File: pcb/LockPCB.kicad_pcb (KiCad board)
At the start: 4 copper layers, 17.5 x 60 mm, 0 parts

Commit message: Record recommended blocker defaults and review envelope
Co-authored-by: arena-agent <297053741+arena-agent@users.noreply.github.com>
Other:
- board text added: "20 x 65 mm REVIEW ENVELOPE - PROPOSED / TBD"
- board text removed: "17.5 x 60 mm - PLACEHOLDER"
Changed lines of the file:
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@@
   (gr_text "BATTERY_CONTACT_ZONE" (at -2.8 21.5 0) (layer "User.2") (effects (font (size 0.62 0.62) (thickness 0.1))))
   (gr_text "CONTACT / POLARITY TBD" (at -2.8 39 0) (layer "User.2") (effects (font (size 0.56 0.56) (thickness 0.09))))
-  (gr_rect (start 0 0) (end 17.5 60) (stroke (width 0.12) (type dash)) (fill none) (layer "User.3"))
+  (gr_rect (start -1.25 -2.5) (end 18.75 62.5) (stroke (width 0.12) (type dash)) (fill none) (layer "User.3"))
   (gr_text "PCB_MAX_OUTLINE" (at 1.0 2.0 0) (layer "User.3") (effects (font (size 0.72 0.72) (thickness 0.11))))
-  (gr_text "17.5 x 60 mm - PLACEHOLDER" (at 1.0 4.0 0) (layer "User.3") (effects (font (size 0.58 0.58) (thickness 0.09))))
+  (gr_text "20 x 65 mm REVIEW ENVELOPE - PROPOSED / TBD" (at 1.0 4.0 0) (layer "User.3") (effects (font (size 0.58 0.58) (thickness 0.09))))
   (gr_rect (start -1 -10) (end 18.5 8) (stroke (width 0.2) (type dash)) (fill none) (layer "User.4"))
   (gr_text "MOTOR_GEARBOX_ZONE" (at -0.2 -8.2 0) (layer "User.4") (effects (font (size 0.72 0.72) (thickness 0.11))))

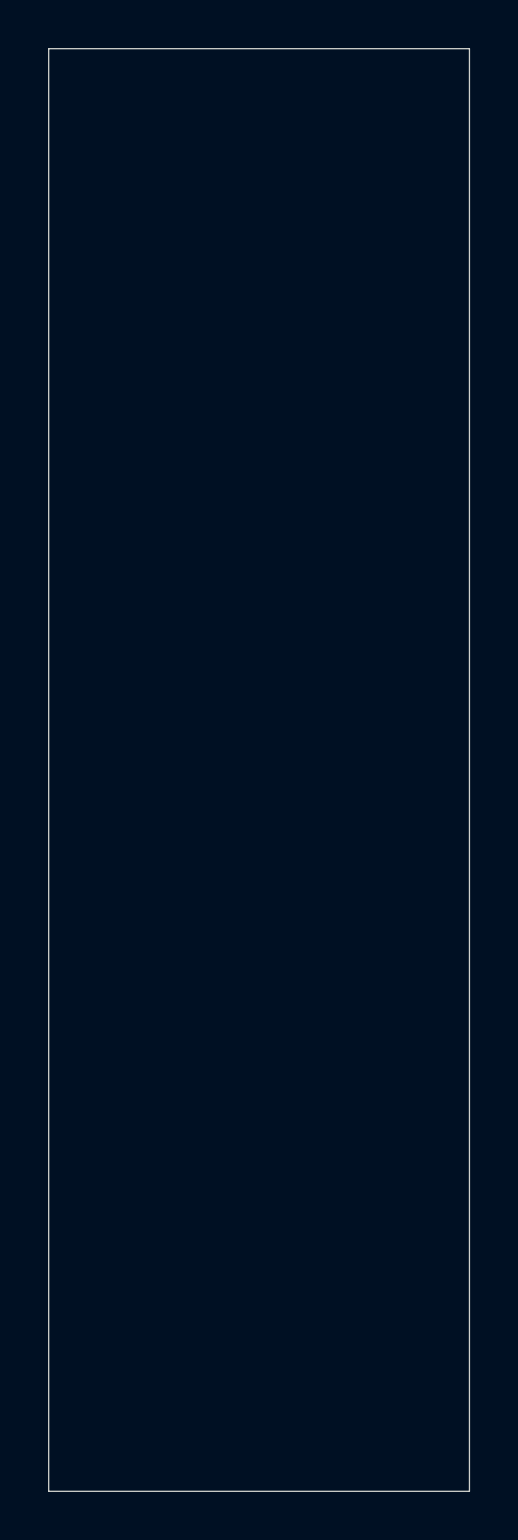
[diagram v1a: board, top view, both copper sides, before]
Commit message: Align agent PCB outline to confirmed prototype CAD
Co-authored-by: arena-agent <297053741+arena-agent@users.noreply.github.com>
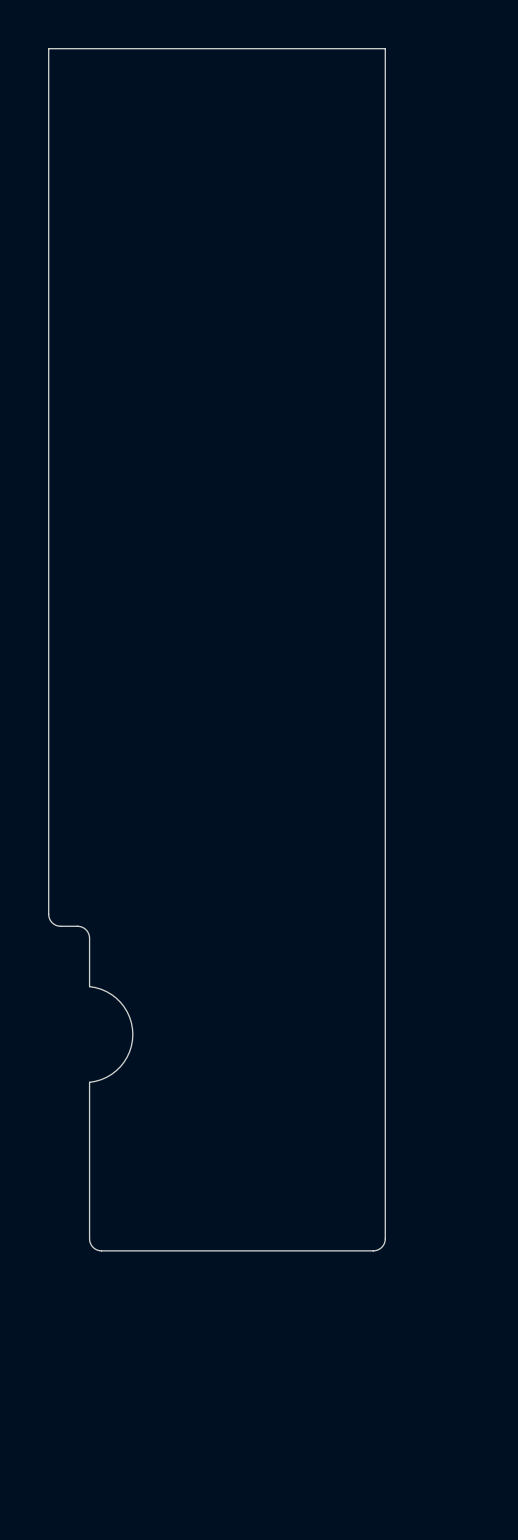
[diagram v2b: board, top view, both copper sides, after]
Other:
- board size 17.5 x 60 mm -> 14 x 50 mm
- board text added: "2x D3.1 / D5 RINGS; PADS / POLARITY TBD"
- board text added: "4-CU PREFERENCE; DWG THICKNESS CALLOUT 1.20 mm; STACKUP TBD"
- board text added: "CELL SKU / CONTACT PAD IMPLEMENTATION / MOTOR DATA / FINAL FIT: TBD"
- board text added: "DESIGNER DWG: 14 x 50 mm; NO EXTRA MARGIN SPECIFIED"
- board text added: "DWG-DERIVED EDGE / HOLE REFERENCES; AGENT ZONES STILL PROVISIONAL - NOT FOR FABRICATION"
- board text added: "PCB_MAX_OUTLINE - SOURCE EXTENT"
- board text added: "STEP 18x50 AABB; ORIENTATION / CLEARANCE TBD"
- board text removed: "18650 SIZE, MOTOR DATA, BODY FIT, CLEARANCES: TBD"
- board text removed: "20 x 65 mm REVIEW ENVELOPE - PROPOSED / TBD"
- board text removed: "4-CU STARTING PREFERENCE; PCB THICKNESS / COPPER WEIGHT: TBD"
- board text removed: "CONTACT / POLARITY TBD"
- board text removed: "MECHANICAL PLACEHOLDERS - NOT TO SCALE - NOT FOR FABRICATION"
- board text removed: "PCB_MAX_OUTLINE"
- board text removed: "TBD / NTS"
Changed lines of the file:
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@@
     (58 "User.9" user)
   )
-  (gr_line (start 0 0) (end 17.5 0) (stroke (width 0.05) (type default)) (layer "Edge.Cuts"))
-  (gr_line (start 17.5 0) (end 17.5 60) (stroke (width 0.05) (type default)) (layer "Edge.Cuts"))
-  (gr_line (start 17.5 60) (end 0 60) (stroke (width 0.05) (type default)) (layer "Edge.Cuts"))
-  (gr_line (start 0 60) (end 0 0) (stroke (width 0.05) (type default)) (layer "Edge.Cuts"))
-  (gr_rect (start -21 1) (end -1 59) (stroke (width 0.18) (type dash)) (fill none) (layer "User.1"))
-  (gr_text "BATTERY_KEEP_OUT" (at -20 0 0) (layer "User.1") (effects (font (size 0.72 0.72) (thickness 0.11))))
-  (gr_text "TBD / NTS" (at -19 3 0) (layer "User.1") (effects (font (size 0.65 0.65) (thickness 0.1))))
-  (gr_rect (start -3 23) (end 0.5 37) (stroke (width 0.2) (type dash)) (fill none) (layer "User.2"))
-  (gr_text "BATTERY_CONTACT_ZONE" (at -2.8 21.5 0) (layer "User.2") (effects (font (size 0.62 0.62) (thickness 0.1))))
-  (gr_text "CONTACT / POLARITY TBD" (at -2.8 39 0) (layer "User.2") (effects (font (size 0.56 0.56) (thickness 0.09))))
-  (gr_rect (start -1.25 -2.5) (end 18.75 62.5) (stroke (width 0.12) (type dash)) (fill none) (layer "User.3"))
-  (gr_text "PCB_MAX_OUTLINE" (at 1.0 2.0 0) (layer "User.3") (effects (font (size 0.72 0.72) (thickness 0.11))))
-  (gr_text "20 x 65 mm REVIEW ENVELOPE - PROPOSED / TBD" (at 1.0 4.0 0) (layer "User.3") (effects (font (size 0.58 0.58) (thickness 0.09))))
+  (gr_line (start 0 0) (end 14 0) (stroke (width 0.05) (type default)) (layer "Edge.Cuts"))
+  (gr_line (start 14 0) (end 14 49.5) (stroke (width 0.05) (type default)) (layer "Edge.Cuts"))
+  (gr_arc (start 14 49.5) (mid 13.853553 49.853553) (end 13.5 50) (stroke (width 0.05) (type default)) (layer "Edge.Cuts"))
+  (gr_line (start 13.5 50) (end 2.2 50) (stroke (width 0.05) (type default)) (layer "Edge.Cuts"))
+  (gr_arc (start 2.2 50) (mid 1.846447 49.853553) (end 1.7 49.5) (stroke (width 0.05) (type default)) (layer "Edge.Cuts"))
+  (gr_line (start 1.7 49.5) (end 1.7 42.99) (stroke (width 0.05) (type default)) (layer "Edge.Cuts"))
+  (gr_arc (start 1.7 42.99) (mid 3.5 41.0) (end 1.7 39.01) (stroke (width 0.05) (type default)) (layer "Edge.Cuts"))
+  (gr_line (start 1.7 39.01) (end 1.7 37.0) (stroke (width 0.05) (type default)) (layer "Edge.Cuts"))
+  (gr_arc (start 1.7 37.0) (mid 1.553553 36.646447) (end 1.2 36.5) (stroke (width 0.05) (type default)) (layer "Edge.Cuts"))
+  (gr_line (start 1.2 36.5) (end 0.5 36.5) (stroke (width 0.05) (type default)) (layer "Edge.Cuts"))
+  (gr_arc (start 0.5 36.5) (mid 0.146447 36.353553) (end 0 36.0) (stroke (width 0.05) (type default)) (layer "Edge.Cuts"))
+  (gr_line (start 0 36.0) (end 0 0) (stroke (width 0.05) (type default)) (layer "Edge.Cuts"))
+  (gr_circle (center 7 10) (end 9.5 10) (stroke (width 0.12) (type default)) (fill none) (layer "Dwgs.User"))
+  (gr_circle (center 7 10) (end 8.55 10) (stroke (width 0.12) (type default)) (fill none) (layer "Dwgs.User"))
+  (gr_circle (center 7 47) (end 9.5 47) (stroke (width 0.12) (type default)) (fill none) (layer "Dwgs.User"))
+  (gr_circle (center 7 47) (end 8.55 47) (stroke (width 0.12) (type default)) (fill none) (layer "Dwgs.User"))
+  (gr_rect (start -18.6 2.5) (end -0.6 52.5) (stroke (width 0.18) (type dash)) (fill none) (layer "User.1"))
+  (gr_text "BATTERY_KEEP_OUT" (at -18 1 0) (layer "User.1") (effects (font (size 0.65 0.65) (thickness 0.1))))
+  (gr_text "STEP 18x50 AABB; ORIENTATION / CLEARANCE TBD" (at -18 4 0) (layer "User.1") (effects (font (size 0.48 0.48) (thickness 0.08))))
+  (gr_text "BATTERY_CONTACT_ZONE" (at 14.8 23 90) (layer "User.2") (effects (font (size 0.55 0.55) (thickness 0.09))))
+  (gr_text "2x D3.1 / D5 RINGS; PADS / POLARITY TBD" (at 15.5 23 90) (layer "User.2") (effects (font (size 0.45 0.45) (thickness 0.075))))
+  (gr_rect (start 0 0) (end 14 50) (stroke (width 0.12) (type dash)) (fill none) (layer "User.3"))
+  (gr_text "PCB_MAX_OUTLINE - SOURCE EXTENT" (at 15 25 90) (layer "User.3") (effects (font (size 0.55 0.55) (thickness 0.09))))
+  (gr_text "DESIGNER DWG: 14 x 50 mm; NO EXTRA MARGIN SPECIFIED" (at 15.7 25 90) (layer "User.3") (effects (font (size 0.43 0.43) (thickness 0.07))))
   (gr_rect (start -1 -10) (end 18.5 8) (stroke (width 0.2) (type dash)) (fill none) (layer "User.4"))
   (gr_text "MOTOR_GEARBOX_ZONE" (at -0.2 -8.2 0) (layer "User.4") (effects (font (size 0.72 0.72) (thickness 0.11))))
@@
   (gr_text "SERVICE_ACCESS_ZONE" (at 2.4 12 0) (layer "User.8") (effects (font (size 0.68 0.68) (thickness 0.1))))
   (gr_text "INTERFACE TBD" (at 2.4 17 0) (layer "User.8") (effects (font (size 0.58 0.58) (thickness 0.09))))
-  (gr_rect (start 0 0) (end 17.5 8) (stroke (width 0.2) (type dash)) (fill none) (layer "User.9"))
+  (gr_rect (start 0 0) (end 14 8) (stroke (width 0.2) (type dash)) (fill none) (layer "User.9"))
   (gr_text "NO_COMPONENT_ZONE" (at 1 7 0) (layer "User.9") (effects (font (size 0.72 0.72) (thickness 0.11))))
   (gr_text "DRIVE / MECH RESERVE - TBD" (at 1 1.3 0) (layer "User.9") (effects (font (size 0.55 0.55) (thickness 0.085))))
-  (gr_text "MECHANICAL PLACEHOLDERS - NOT TO SCALE - NOT FOR FABRICATION" (at -22 66 0) (layer "Cmts.User") (effects (font (size 0.8 0.8) (thickness 0.12))))
+  (gr_text "DWG-DERIVED EDGE / HOLE REFERENCES; AGENT ZONES STILL PROVISIONAL - NOT FOR FABRICATION" (at -22 66 0) (layer "Cmts.User") (effects (font (size 0.62 0.62) (thickness 0.1))))
   (gr_text "NO COMPONENTS / NO COPPER / NO ROUTING / NOT READY FOR FAB" (at -22 68.5 0) (layer "Cmts.User") (effects (font (size 0.7 0.7) (thickness 0.11))))
-  (gr_text "18650 SIZE, MOTOR DATA, BODY FIT, CLEARANCES: TBD" (at -22 71 0) (layer "Cmts.User") (effects (font (size 0.7 0.7) (thickness 0.11))))
-  (gr_text "4-CU STARTING PREFERENCE; PCB THICKNESS / COPPER WEIGHT: TBD" (at -22 73.5 0) (layer "Cmts.User") (effects (font (size 0.7 0.7) (thickness 0.11))))
+  (gr_text "CELL SKU / CONTACT PAD IMPLEMENTATION / MOTOR DATA / FINAL FIT: TBD" (at -22 71 0) (layer "Cmts.User") (effects (font (size 0.62 0.62) (thickness 0.1))))
+  (gr_text "4-CU PREFERENCE; DWG THICKNESS CALLOUT 1.20 mm; STACKUP TBD" (at -22 73.5 0) (layer "Cmts.User") (effects (font (size 0.62 0.62) (thickness 0.1))))
   (gr_rect (start 0.5 9) (end 17 23) (stroke (width 0.18) (type dash)) (fill none) (layer "Eco1.User"))
   (gr_text "MOTOR_CURRENT_ZONE - PLACEHOLDER" (at 0.8 11 0) (layer "Eco1.User") (effects (font (size 0.6 0.6) (thickness 0.1))))
@@
   (gr_text "RF_SENSITIVE_ZONE - PLACEHOLDER" (at 0.8 44 0) (layer "Eco2.User") (effects (font (size 0.6 0.6) (thickness 0.1))))
   (gr_text "ANTENNA / METAL CLEARANCE TBD" (at 0.8 55 0) (layer "Eco2.User") (effects (font (size 0.55 0.55) (thickness 0.09))))
-  (zone (net 0) (net_name "") (layers "F.Cu" "In1.Cu" "In2.Cu" "B.Cu") (name "NO_COMPONENT_ZONE_PLACEHOLDER") (hatch edge 0.5) (connect_pads (clearance 0)) (min_thickness 0.25) (keepout (tracks not_allowed) (vias not_allowed) (pads not_allowed) (copperpour not_allowed) (footprints not_allowed)) (polygon (pts (xy 0 0) (xy 17.5 0) (xy 17.5 8) (xy 0 8))))
+  (zone (net 0) (net_name "") (layers "F.Cu" "In1.Cu" "In2.Cu" "B.Cu") (name "NO_COMPONENT_ZONE_PLACEHOLDER") (hatch edge 0.5) (connect_pads (clearance 0)) (min_thickness 0.25) (keepout (tracks not_allowed) (vias not_allowed) (pads not_allowed) (copperpour not_allowed) (footprints not_allowed)) (polygon (pts (xy 0 0) (xy 14 0) (xy 14 8) (xy 0 8))))
 )

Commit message: Set V1 PCB target to 18650 variant
Co-authored-by: arena-agent <297053741+arena-agent@users.noreply.github.com>
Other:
- board text added: "V1 18650 ENVELOPE 19x70 PROVISIONAL; VERIFY SKU / FIT"
- board text added: "V1 18650 TARGET; CELL SKU / CONTACTS / MOTOR / FINAL FIT: TBD"
- board text removed: "CELL SKU / CONTACT PAD IMPLEMENTATION / MOTOR DATA / FINAL FIT: TBD"
- board text removed: "STEP 18x50 AABB; ORIENTATION / CLEARANCE TBD"
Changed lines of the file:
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@@
   (gr_circle (center 7 47) (end 9.5 47) (stroke (width 0.12) (type default)) (fill none) (layer "Dwgs.User"))
   (gr_circle (center 7 47) (end 8.55 47) (stroke (width 0.12) (type default)) (fill none) (layer "Dwgs.User"))
-  (gr_rect (start -18.6 2.5) (end -0.6 52.5) (stroke (width 0.18) (type dash)) (fill none) (layer "User.1"))
+  (gr_rect (start -19.6 2.5) (end -0.6 72.5) (stroke (width 0.18) (type dash)) (fill none) (layer "User.1"))
   (gr_text "BATTERY_KEEP_OUT" (at -18 1 0) (layer "User.1") (effects (font (size 0.65 0.65) (thickness 0.1))))
-  (gr_text "STEP 18x50 AABB; ORIENTATION / CLEARANCE TBD" (at -18 4 0) (layer "User.1") (effects (font (size 0.48 0.48) (thickness 0.08))))
+  (gr_text "V1 18650 ENVELOPE 19x70 PROVISIONAL; VERIFY SKU / FIT" (at -18 4 0) (layer "User.1") (effects (font (size 0.48 0.48) (thickness 0.08))))
   (gr_text "BATTERY_CONTACT_ZONE" (at 14.8 23 90) (layer "User.2") (effects (font (size 0.55 0.55) (thickness 0.09))))
   (gr_text "2x D3.1 / D5 RINGS; PADS / POLARITY TBD" (at 15.5 23 90) (layer "User.2") (effects (font (size 0.45 0.45) (thickness 0.075))))
@@
   (gr_text "DWG-DERIVED EDGE / HOLE REFERENCES; AGENT ZONES STILL PROVISIONAL - NOT FOR FABRICATION" (at -22 66 0) (layer "Cmts.User") (effects (font (size 0.62 0.62) (thickness 0.1))))
   (gr_text "NO COMPONENTS / NO COPPER / NO ROUTING / NOT READY FOR FAB" (at -22 68.5 0) (layer "Cmts.User") (effects (font (size 0.7 0.7) (thickness 0.11))))
-  (gr_text "CELL SKU / CONTACT PAD IMPLEMENTATION / MOTOR DATA / FINAL FIT: TBD" (at -22 71 0) (layer "Cmts.User") (effects (font (size 0.62 0.62) (thickness 0.1))))
+  (gr_text "V1 18650 TARGET; CELL SKU / CONTACTS / MOTOR / FINAL FIT: TBD" (at -22 71 0) (layer "Cmts.User") (effects (font (size 0.62 0.62) (thickness 0.1))))
   (gr_text "4-CU PREFERENCE; DWG THICKNESS CALLOUT 1.20 mm; STACKUP TBD" (at -22 73.5 0) (layer "Cmts.User") (effects (font (size 0.62 0.62) (thickness 0.1))))
   (gr_rect (start 0.5 9) (end 17 23) (stroke (width 0.18) (type dash)) (fill none) (layer "Eco1.User"))
